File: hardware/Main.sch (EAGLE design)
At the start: 90 parts, among them IC1 ESP32-WROOM-32D_M113DH3200PH3Q, IC2 LAN8720A-CP-ABC, IC3 R-78E5.0-1.0, IC4 LT1129MPST-3.3#PBF, J2 1727078, J3 HR911105A, J4 1727010, J5 1727049, J6 1727049, Q1 O50.0-JO32-B-3.3-1, Q10 BSS123, Q11 BSS123, Q12 BSS123, Q2 IPD031N06L3GATMA1, Q3 IPD031N06L3GATMA1, Q4 IPD031N06L3GATMA1, Q5 IPD031N06L3GATMA1, Q6 IPD031N06L3GATMA1, Q7 BSS123, Q8 BSS123, Q9 BSS123

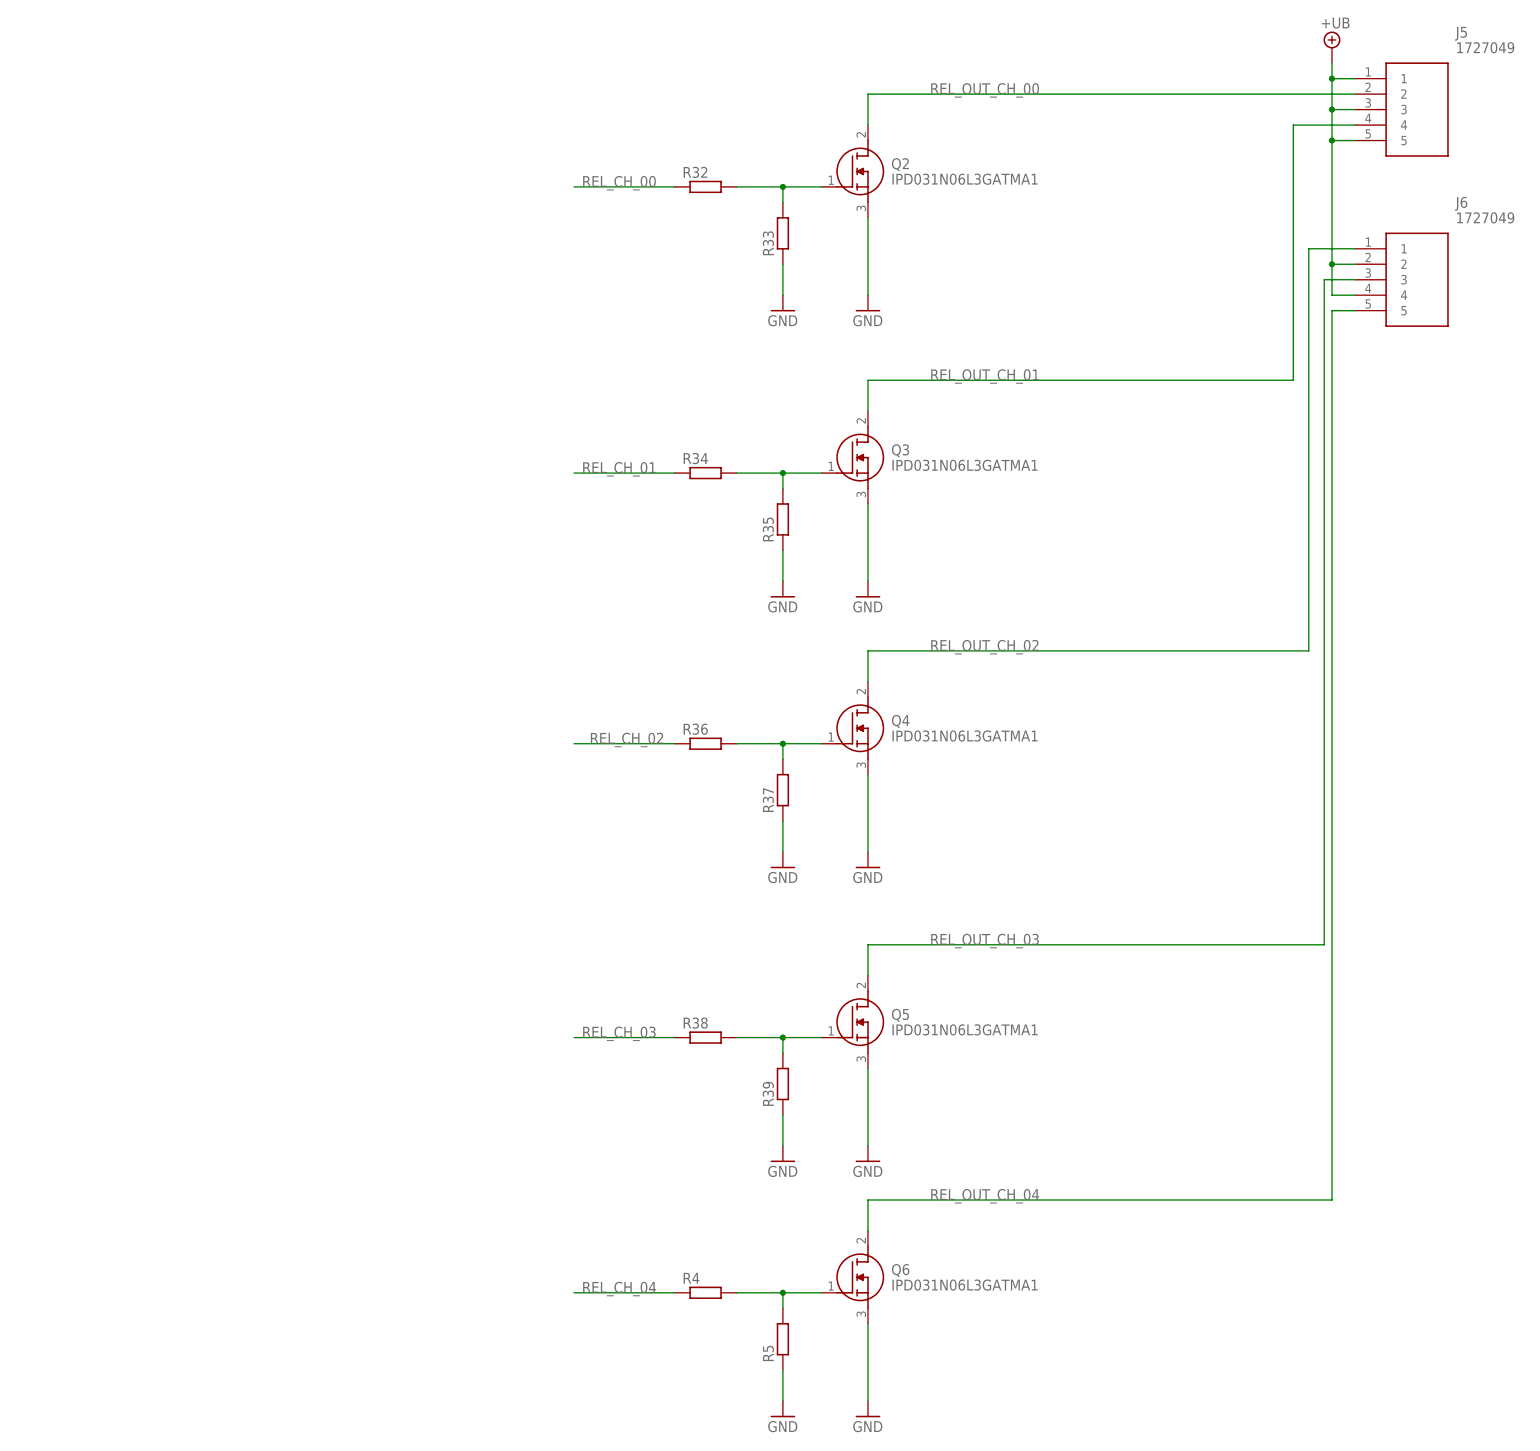
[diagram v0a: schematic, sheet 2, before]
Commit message: Layout fertig
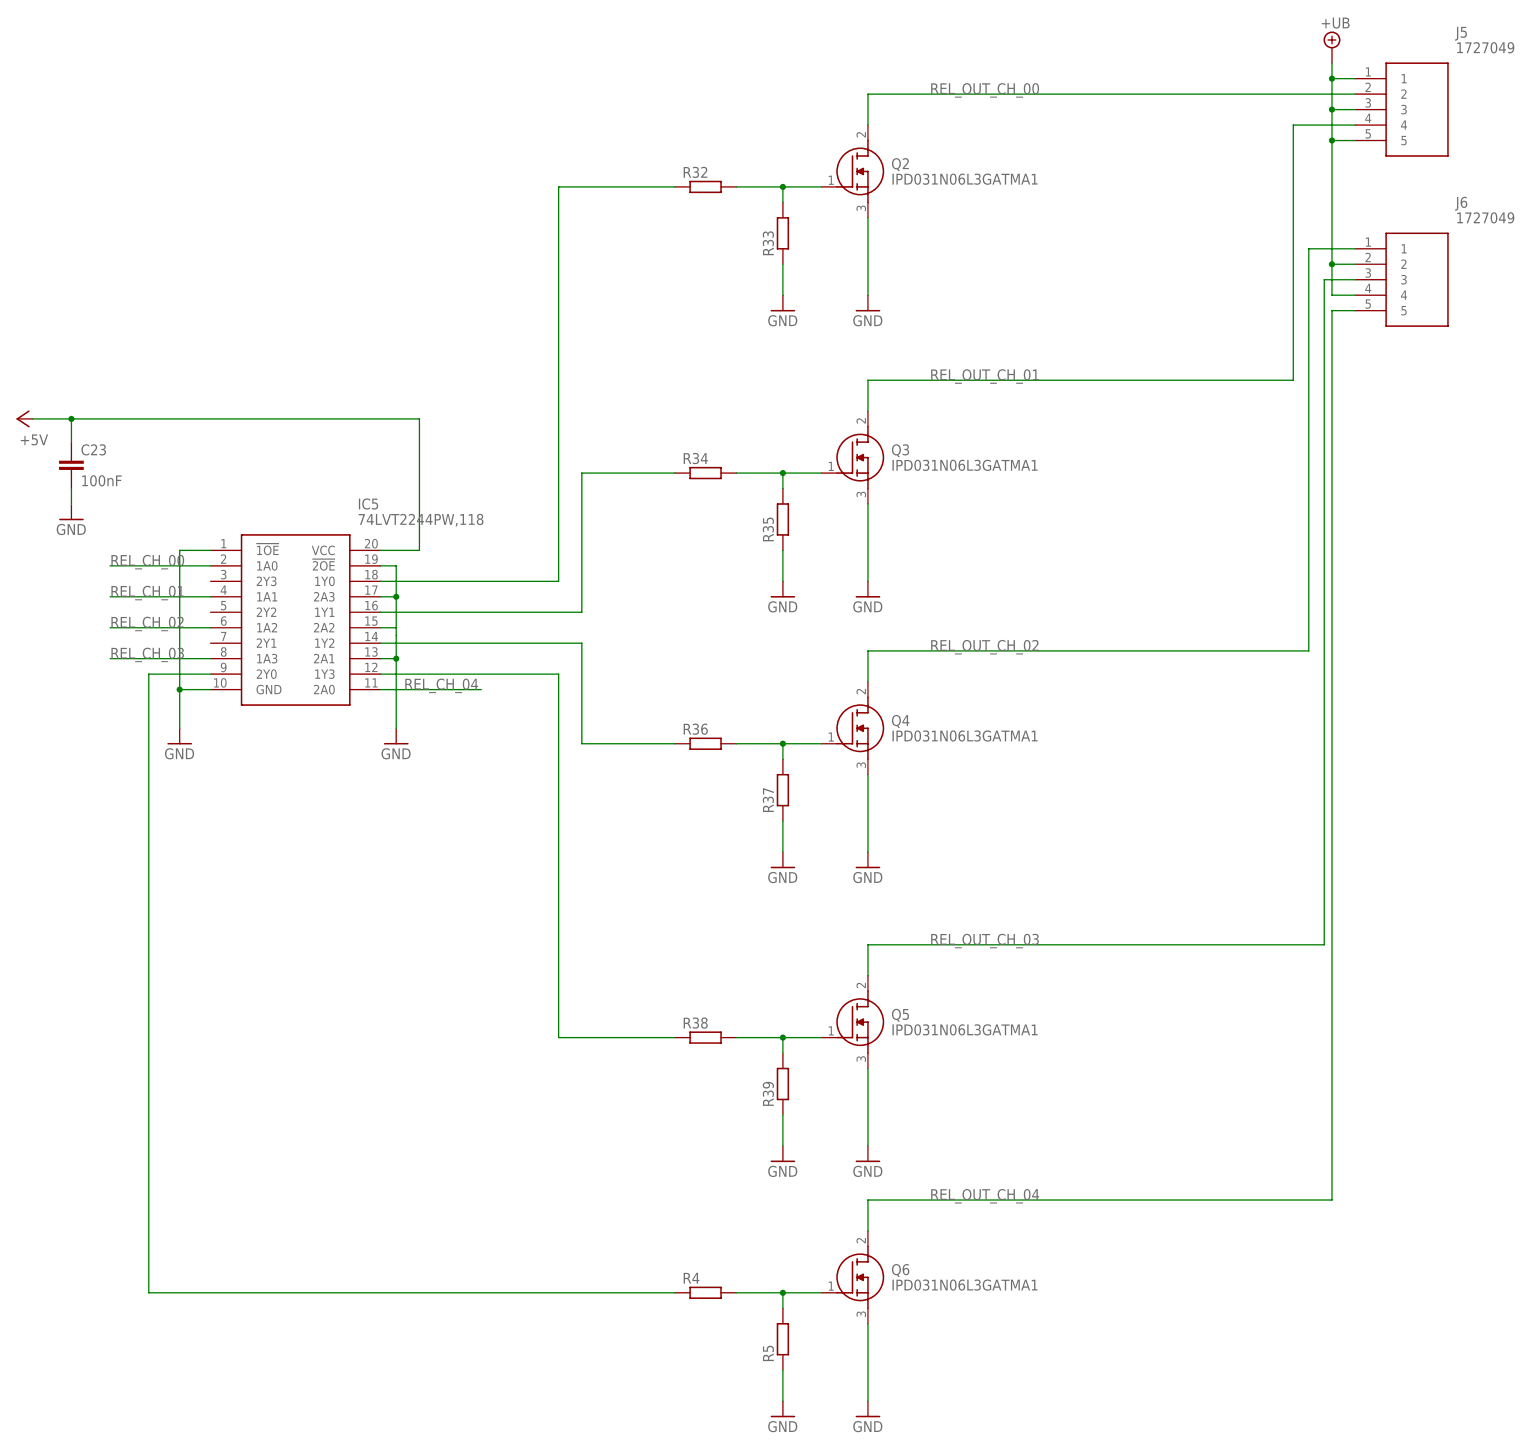
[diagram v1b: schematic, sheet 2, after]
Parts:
- added C23: 100nF, rcl:C-EUC0603
- added IC5: 74LVT2244PW,118, SamacSys_Parts:74LVT2244PW,118
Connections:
- new net N$1: IC5.1Y0, R32.1
- new net N$10: IC5.1Y2, R36.1
- new net N$17: IC5.1Y3, R38.1
- new net N$32: IC5.2Y0, R4.1
- new net N$7: IC5.1Y1, R34.1
- net +5V: now also C23.1, IC5.VCC
- net GND: now also C23.2, IC5.!1OE, IC5.!2OE, IC5.2A1, IC5.2A2, IC5.2A3, IC5.GND
- net REL_CH_00: now also IC5.1A0; no longer R32.1
- net REL_CH_01: now also IC5.1A1; no longer R34.1
- net REL_CH_02: now also IC5.1A2; no longer R36.1
- net REL_CH_03: now also IC5.1A3; no longer R38.1
- net REL_CH_04: now also IC5.2A0; no longer R4.1
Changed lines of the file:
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@@
 <part name="GND46" library="supply1" library_urn="urn:adsk.eagle:library:371" deviceset="GND" device=""/>
 <part name="C22" library="rcl" library_urn="urn:adsk.eagle:library:334" deviceset="C-EU" device="C0603" package3d_urn="urn:adsk.eagle:package:23616/2" value="10U/6,3V"/>
+<part name="IC5" library="SamacSys_Parts" deviceset="74LVT2244PW,118" device=""/>
+<part name="GND47" library="supply1" library_urn="urn:adsk.eagle:library:371" deviceset="GND" device=""/>
+<part name="C23" library="rcl" library_urn="urn:adsk.eagle:library:334" deviceset="C-EU" device="C0603" package3d_urn="urn:adsk.eagle:package:23616/2" value="100nF"/>
+<part name="P+6" library="supply1" library_urn="urn:adsk.eagle:library:371" deviceset="+5V" device=""/>
+<part name="GND48" library="supply1" library_urn="urn:adsk.eagle:library:371" deviceset="GND" device=""/>
+<part name="GND49" library="supply1" library_urn="urn:adsk.eagle:library:371" deviceset="GND" device=""/>
 </parts>
 <sheets>
@@
 <attribute name="VALUE" x="271.78" y="214.63" size="1.778" layer="96" align="center-left"/>
 </instance>
+<instance part="IC5" gate="G$1" x="67.31" y="160.02" smashed="yes">
+<attribute name="NAME" x="91.44" y="167.64" size="1.778" layer="95" align="center-left"/>
+<attribute name="VALUE" x="91.44" y="165.1" size="1.778" layer="96" align="center-left"/>
+</instance>
+<instance part="GND47" gate="1" x="44.45" y="165.1" smashed="yes">
+<attribute name="VALUE" x="41.91" y="162.56" size="1.778" layer="96"/>
+</instance>
+<instance part="C23" gate="G$1" x="44.45" y="175.26" smashed="yes">
+<attribute name="NAME" x="45.974" y="175.641" size="1.778" layer="95"/>
+<attribute name="VALUE" x="45.974" y="170.561" size="1.778" layer="96"/>
+</instance>
+<instance part="P+6" gate="1" x="35.56" y="181.61" smashed="yes" rot="R90">
+<attribute name="VALUE" x="40.64" y="179.07" size="1.778" layer="96" rot="R180"/>
+</instance>
+<instance part="GND48" gate="1" x="62.23" y="128.27" smashed="yes">
+<attribute name="VALUE" x="59.69" y="125.73" size="1.778" layer="96"/>
+</instance>
+<instance part="GND49" gate="1" x="97.79" y="128.27" smashed="yes">
+<attribute name="VALUE" x="95.25" y="125.73" size="1.778" layer="96"/>
+</instance>
 </instances>
 <busses>
@@
 <pinref part="R5" gate="G$1" pin="1"/>
 <wire x1="161.29" y1="20.32" x2="161.29" y2="25.4" width="0.1524" layer="91"/>
+</segment>
+<segment>
+<pinref part="GND47" gate="1" pin="GND"/>
+<pinref part="C23" gate="G$1" pin="2"/>
+<wire x1="44.45" y1="167.64" x2="44.45" y2="170.18" width="0.1524" layer="91"/>
+</segment>
+<segment>
+<pinref part="IC5" gate="G$1" pin="GND"/>
+<wire x1="67.31" y1="137.16" x2="62.23" y2="137.16" width="0.1524" layer="91"/>
+<wire x1="62.23" y1="137.16" x2="62.23" y2="130.81" width="0.1524" layer="91"/>
+<pinref part="IC5" gate="G$1" pin="!1OE"/>
+<wire x1="67.31" y1="160.02" x2="62.23" y2="160.02" width="0.1524" layer="91"/>
+<wire x1="62.23" y1="160.02" x2="62.23" y2="137.16" width="0.1524" layer="91"/>
+<junction x="62.23" y="137.16"/>
+<pinref part="GND48" gate="1" pin="GND"/>
+</segment>
+<segment>
+<pinref part="IC5" gate="G$1" pin="2A1"/>
+<wire x1="95.25" y1="142.24" x2="97.79" y2="142.24" width="0.1524" layer="91"/>
+<wire x1="97.79" y1="142.24" x2="97.79" y2="130.81" width="0.1524" layer="91"/>
+<pinref part="IC5" gate="G$1" pin="!2OE"/>
+<wire x1="95.25" y1="157.48" x2="97.79" y2="157.48" width="0.1524" layer="91"/>
+<wire x1="97.79" y1="157.48" x2="97.79" y2="152.4" width="0.1524" layer="91"/>
+<junction x="97.79" y="142.24"/>
+<pinref part="IC5" gate="G$1" pin="2A3"/>
+<wire x1="97.79" y1="152.4" x2="97.79" y2="147.32" width="0.1524" layer="91"/>
+<wire x1="97.79" y1="146.05" x2="97.79" y2="142.24" width="0.1524" layer="91"/>
+<wire x1="95.25" y1="152.4" x2="97.79" y2="152.4" width="0.1524" layer="91"/>
+<junction x="97.79" y="152.4"/>
+<pinref part="IC5" gate="G$1" pin="2A2"/>
+<wire x1="95.25" y1="147.32" x2="97.79" y2="147.32" width="0.1524" layer="91"/>
+<wire x1="97.79" y1="147.32" x2="97.79" y2="146.05" width="0.1524" layer="91"/>
+<pinref part="GND49" gate="1" pin="GND"/>
 </segment>
 </net>
@@
 </segment>
 </net>
-<net name="REL_CH_00" class="0">
-<segment>
-<pinref part="R32" gate="G$1" pin="1"/>
-<wire x1="143.51" y1="219.71" x2="127" y2="219.71" width="0.1524" layer="91"/>
-<label x="128.27" y="219.71" size="1.778" layer="95"/>
-</segment>
-</net>
 <net name="N$15" class="0">
 <segment>
@@
 <net name="REL_CH_01" class="0">
 <segment>
-<pinref part="R34" gate="G$1" pin="1"/>
-<wire x1="143.51" y1="172.72" x2="127" y2="172.72" width="0.1524" layer="91"/>
-<label x="128.27" y="172.72" size="1.778" layer="95"/>
+<label x="50.8" y="152.4" size="1.778" layer="95"/>
+<wire x1="67.31" y1="152.4" x2="50.8" y2="152.4" width="0.1524" layer="91"/>
+<pinref part="IC5" gate="G$1" pin="1A1"/>
 </segment>
 </net>
@@
 <net name="REL_CH_02" class="0">
 <segment>
-<pinref part="R36" gate="G$1" pin="1"/>
-<wire x1="143.51" y1="128.27" x2="127" y2="128.27" width="0.1524" layer="91"/>
-<label x="129.54" y="128.27" size="1.778" layer="95"/>
+<label x="50.8" y="147.32" size="1.778" layer="95"/>
+<wire x1="67.31" y1="147.32" x2="50.8" y2="147.32" width="0.1524" layer="91"/>
+<pinref part="IC5" gate="G$1" pin="1A2"/>
 </segment>
 </net>
@@
 <net name="REL_CH_03" class="0">
 <segment>
-<pinref part="R38" gate="G$1" pin="1"/>
-<wire x1="143.51" y1="80.01" x2="127" y2="80.01" width="0.1524" layer="91"/>
-<label x="128.27" y="80.01" size="1.778" layer="95"/>
+<label x="50.8" y="142.24" size="1.778" layer="95"/>
+<wire x1="67.31" y1="142.24" x2="50.8" y2="142.24" width="0.1524" layer="91"/>
+<pinref part="IC5" gate="G$1" pin="1A3"/>
 </segment>
 </net>
@@
 </segment>
 </net>
+<net name="+5V" class="0">
+<segment>
+<pinref part="C23" gate="G$1" pin="1"/>
+<wire x1="44.45" y1="177.8" x2="44.45" y2="181.61" width="0.1524" layer="91"/>
+<pinref part="P+6" gate="1" pin="+5V"/>
+<wire x1="38.1" y1="181.61" x2="44.45" y2="181.61" width="0.1524" layer="91"/>
+<junction x="44.45" y="181.61"/>
+<pinref part="IC5" gate="G$1" pin="VCC"/>
+<wire x1="95.25" y1="160.02" x2="101.6" y2="160.02" width="0.1524" layer="91"/>
+<wire x1="101.6" y1="160.02" x2="101.6" y2="181.61" width="0.1524" layer="91"/>
+<wire x1="101.6" y1="181.61" x2="44.45" y2="181.61" width="0.1524" layer="91"/>
+</segment>
+</net>
+<net name="REL_CH_00" class="0">
+<segment>
+<wire x1="67.31" y1="157.48" x2="50.8" y2="157.48" width="0.1524" layer="91"/>
+<label x="50.8" y="157.48" size="1.778" layer="95"/>
+<pinref part="IC5" gate="G$1" pin="1A0"/>
+</segment>
+</net>
+<net name="N$1" class="0">
+<segment>
+<pinref part="IC5" gate="G$1" pin="1Y0"/>
+<wire x1="95.25" y1="154.94" x2="124.46" y2="154.94" width="0.1524" layer="91"/>
+<pinref part="R32" gate="G$1" pin="1"/>
+<wire x1="124.46" y1="154.94" x2="124.46" y2="219.71" width="0.1524" layer="91"/>
+<wire x1="124.46" y1="219.71" x2="143.51" y2="219.71" width="0.1524" layer="91"/>
+</segment>
+</net>
+<net name="N$7" class="0">
+<segment>
+<pinref part="IC5" gate="G$1" pin="1Y1"/>
+<wire x1="95.25" y1="149.86" x2="128.27" y2="149.86" width="0.1524" layer="91"/>
+<pinref part="R34" gate="G$1" pin="1"/>
+<wire x1="128.27" y1="149.86" x2="128.27" y2="172.72" width="0.1524" layer="91"/>
+<wire x1="128.27" y1="172.72" x2="143.51" y2="172.72" width="0.1524" layer="91"/>
+</segment>
+</net>
+<net name="N$10" class="0">
+<segment>
+<pinref part="IC5" gate="G$1" pin="1Y2"/>
+<wire x1="95.25" y1="144.78" x2="128.27" y2="144.78" width="0.1524" layer="91"/>
+<pinref part="R36" gate="G$1" pin="1"/>
+<wire x1="128.27" y1="144.78" x2="128.27" y2="128.27" width="0.1524" layer="91"/>
+<wire x1="128.27" y1="128.27" x2="143.51" y2="128.27" width="0.1524" layer="91"/>
+</segment>
+</net>
+<net name="N$17" class="0">
+<segment>
+<pinref part="IC5" gate="G$1" pin="1Y3"/>
+<wire x1="95.25" y1="139.7" x2="124.46" y2="139.7" width="0.1524" layer="91"/>
+<wire x1="124.46" y1="139.7" x2="124.46" y2="80.01" width="0.1524" layer="91"/>
+<pinref part="R38" gate="G$1" pin="1"/>
+<wire x1="124.46" y1="80.01" x2="143.51" y2="80.01" width="0.1524" layer="91"/>
+</segment>
+</net>
+<net name="N$32" class="0">
+<segment>
+<pinref part="IC5" gate="G$1" pin="2Y0"/>
+<wire x1="67.31" y1="139.7" x2="57.15" y2="139.7" width="0.1524" layer="91"/>
+<wire x1="57.15" y1="139.7" x2="57.15" y2="38.1" width="0.1524" layer="91"/>
+<wire x1="57.15" y1="38.1" x2="143.51" y2="38.1" width="0.1524" layer="91"/>
+<pinref part="R4" gate="G$1" pin="1"/>
+</segment>
+</net>
 <net name="REL_CH_04" class="0">
 <segment>
-<pinref part="R4" gate="G$1" pin="1"/>
-<wire x1="143.51" y1="38.1" x2="127" y2="38.1" width="0.1524" layer="91"/>
-<label x="128.27" y="38.1" size="1.778" layer="95"/>
-</segment>
-</net>
+<wire x1="111.76" y1="137.16" x2="95.25" y2="137.16" width="0.1524" layer="91"/>
+<label x="99.06" y="137.16" size="1.778" layer="95"/>
+<pinref part="IC5" gate="G$1" pin="2A0"/>
+</segment>
+</net>
